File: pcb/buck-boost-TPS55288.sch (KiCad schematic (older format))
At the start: 19 parts, among them Q201 Q_DUAL_NMOS_G1S2G2D2S1D1, U201 TPS55288RPM

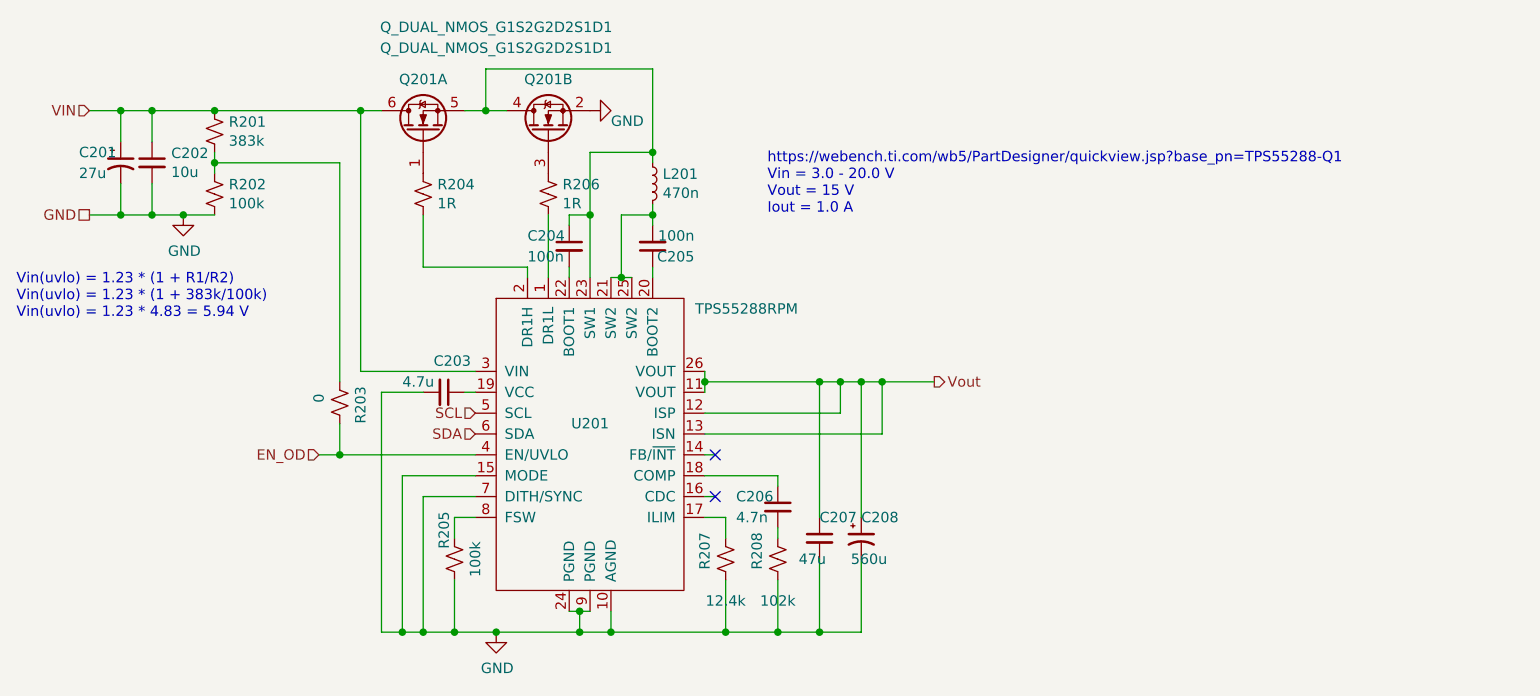
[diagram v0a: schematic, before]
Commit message: [PCB] minor changes
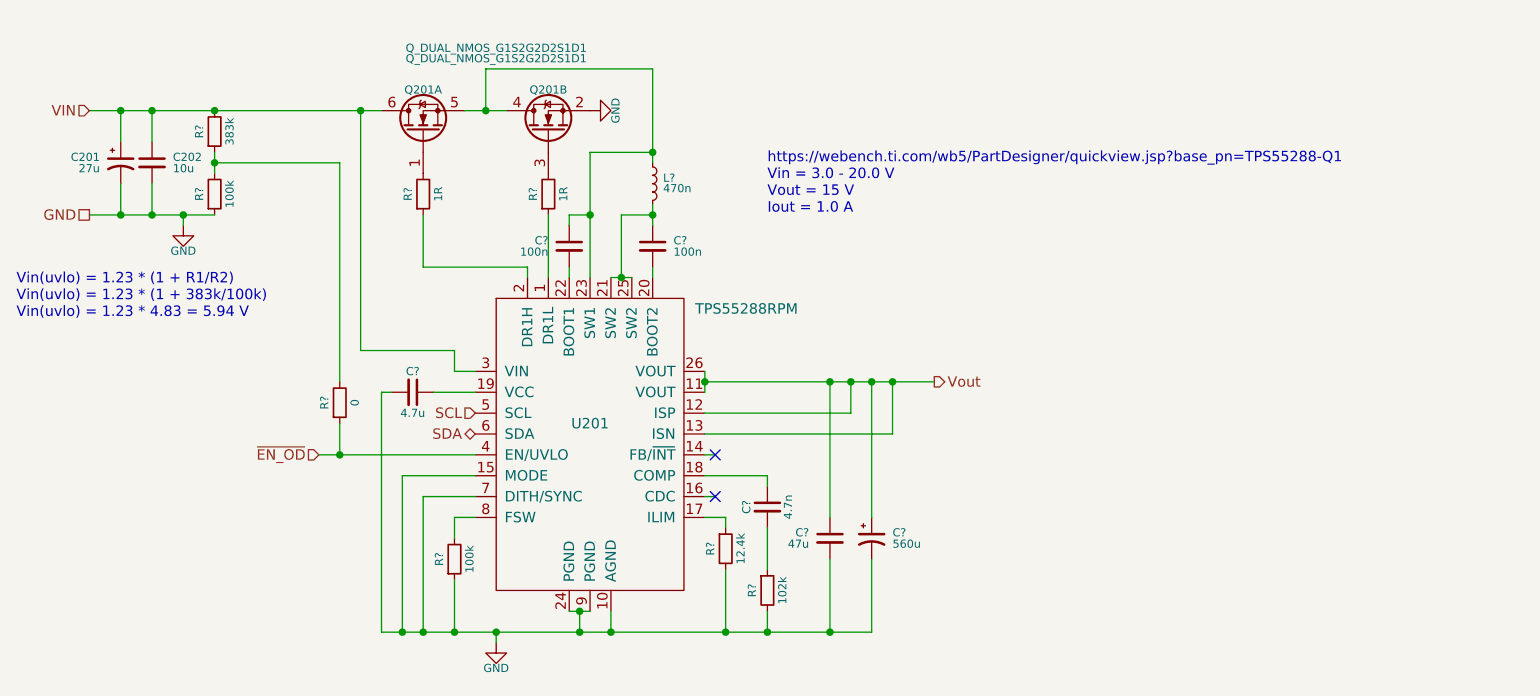
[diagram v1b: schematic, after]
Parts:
- removed C203: 4.7u, symbol Device:C_Small
- removed C204, C205: 100n, symbol Device:C_Small
- removed C206: 4.7n, symbol Device:C_Small
- removed C207: 47u, symbol Device:C_Small
- removed C208: 560u, symbol Device:CP1_Small
- removed L201: 470n, symbol Device:L_Small
- removed R201: 383k, symbol Device:R_Small_US
- removed R202, R205: 100k, symbol Device:R_Small_US
- removed R203: 0, symbol Device:R_Small_US
- removed R204, R206: 1R, symbol Device:R_Small_US
- removed R207: 12.4k, symbol Device:R_Small_US
- removed R208: 102k, symbol Device:R_Small_US
- added C?: 4.7u, Capacitor_SMD:C_0603_1608Metric, symbol Device:C_Small
- added C?: 4.7n, Capacitor_SMD:C_0603_1608Metric, symbol Device:C_Small
- added C?: 47u, Capacitor_SMD:C_0603_1608Metric, symbol Device:C_Small
- added C?: 560u, Capacitor_SMD:C_0603_1608Metric, symbol Device:CP1_Small
- added C? (x2): 100n, Capacitor_SMD:C_0603_1608Metric, symbol Device:C_Small
- added L?: 470n, symbol Device:L_Small
- added R?: 383k, symbol Device:R_Small
- added R? (x2): 100k, symbol Device:R_Small
- added R? (x2): 1R, symbol Device:R_Small
- added R?: 0, symbol Device:R_Small
- added R?: 12.4k, symbol Device:R_Small
- added R?: 102k, symbol Device:R_Small
- C201, C202: footprint (none) -> Capacitor_SMD:C_0603_1608Metric
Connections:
- net GND: now also C?.2, C?.2, C?.2, R?.1, R?.1, R?.2, R?.2
- net VIN: now also R?.2
- net Vout: now also C?.1, C?.1
- net at U201.1 (DR1L): now also R?.1
- net at U201.17 (ILIM): now also R?.1
- net at U201.18 (COMP): now also C?.1
- net at U201.19 (VCC): now also C?.1
- net at U201.2 (DR1H): now also R?.1
- net at U201.20 (BOOT2): now also C?.2
- net at U201.21 (SW2), U201.25 (SW2): now also C?.1, L?.2
- net at U201.22 (BOOT1): now also C?.2
- net at Q201.4 (D), Q201.5 (S), U201.23 (SW1): now also C?.1, L?.1
- net at U201.8 (FSW): now also R?.2
- net at Q201.1 (G): now also R?.2
- net at Q201.3 (G): now also R?.2
- net EN_OD renamed ~EN_OD
- net ~EN_OD: now also R?.1
- new net: R?.1, R?.2, R?.2
- new net: C?.2, R?.1
